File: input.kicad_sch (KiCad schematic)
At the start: 11 parts, among them J1 Conn_01x08

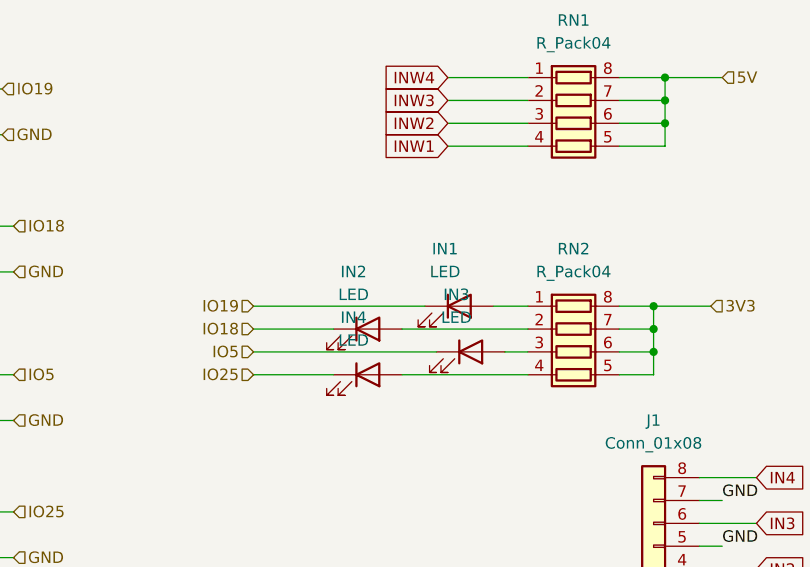
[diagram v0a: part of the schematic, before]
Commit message: 0
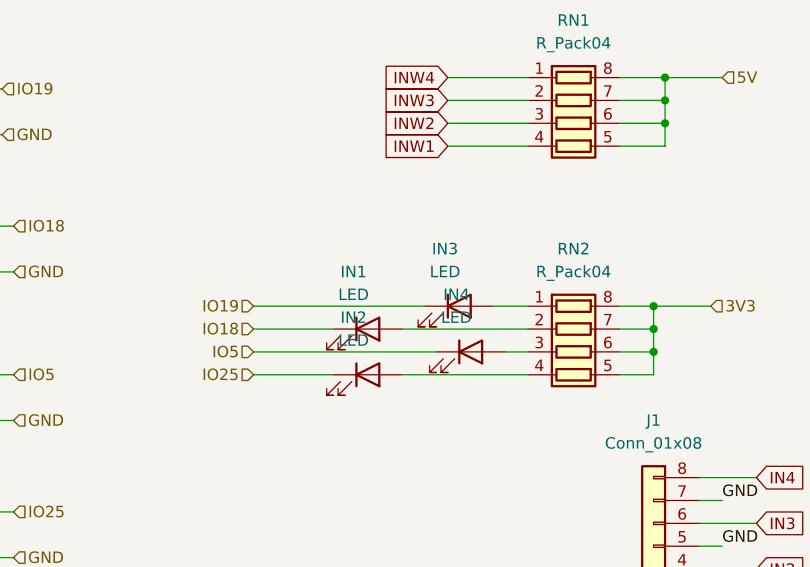
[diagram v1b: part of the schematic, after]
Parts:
- renumbered IN2 to IN1, IN4 to IN2, IN1 to IN3, IN3 to IN4
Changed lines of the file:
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@@
 		(pin "1"
+		)
+		(instances
+			(project "electronica"
+				(path "/a1c80da3-9403-4ec6-a34a-1db23a22b009/5b7b1883-0956-4642-a84a-0fce661aecfc"
+					(reference "OPT4")
+					(unit 1)
+				)
+			)
 		)
 	)
@@
 		(pin "1"
 		)
+		(instances
+			(project "electronica"
+				(path "/a1c80da3-9403-4ec6-a34a-1db23a22b009/5b7b1883-0956-4642-a84a-0fce661aecfc"
+					(reference "J1")
+					(unit 1)
+				)
+			)
+		)
 	)
 	(symbol
@@
 		(pin "8"
 		)
+		(instances
+			(project "electronica"
+				(path "/a1c80da3-9403-4ec6-a34a-1db23a22b009/5b7b1883-0956-4642-a84a-0fce661aecfc"
+					(reference "RN2")
+					(unit 1)
+				)
+			)
+		)
 	)
 	(symbol
@@
 		(pin "1"
 		)
+		(instances
+			(project "electronica"
+				(path "/a1c80da3-9403-4ec6-a34a-1db23a22b009/5b7b1883-0956-4642-a84a-0fce661aecfc"
+					(reference "OPT2")
+					(unit 1)
+				)
+			)
+		)
 	)
 	(symbol
@@
 		(pin "1"
 		)
+		(instances
+			(project "electronica"
+				(path "/a1c80da3-9403-4ec6-a34a-1db23a22b009/5b7b1883-0956-4642-a84a-0fce661aecfc"
+					(reference "OPT3")
+					(unit 1)
+				)
+			)
+		)
 	)
 	(symbol
@@
 		(dnp no)
 		(fields_autoplaced yes)
-		(property "Reference" "IN4"
+		(property "Reference" "IN2"
 			(at 171.1325 106.68 0)
 			(effects
@@
 		(pin "1"
 		)
+		(instances
+			(project "electronica"
+				(path "/a1c80da3-9403-4ec6-a34a-1db23a22b009/5b7b1883-0956-4642-a84a-0fce661aecfc"
+					(reference "IN2")
+					(unit 1)
+				)
+			)
+		)
 	)
 	(symbol
@@
 		(dnp no)
 		(fields_autoplaced yes)
-		(property "Reference" "IN1"
+		(property "Reference" "IN3"
 			(at 181.2925 99.06 0)
 			(effects
@@
 		(pin "1"
 		)
+		(instances
+			(project "electronica"
+				(path "/a1c80da3-9403-4ec6-a34a-1db23a22b009/5b7b1883-0956-4642-a84a-0fce661aecfc"
+					(reference "IN3")
+					(unit 1)
+				)
+			)
+		)
 	)
 	(symbol
@@
 		(dnp no)
 		(fields_autoplaced yes)
-		(property "Reference" "IN3"
+		(property "Reference" "IN4"
 			(at 182.5625 104.14 0)
 			(effects
@@
 		(pin "1"
 		)
+		(instances
+			(project "electronica"
+				(path "/a1c80da3-9403-4ec6-a34a-1db23a22b009/5b7b1883-0956-4642-a84a-0fce661aecfc"
+					(reference "IN4")
+					(unit 1)
+				)
+			)
+		)
 	)
 	(symbol
@@
 		(dnp no)
 		(fields_autoplaced yes)
-		(property "Reference" "IN2"
+		(property "Reference" "IN1"
 			(at 171.1325 101.6 0)
 			(effects
@@
 		(pin "1"
 		)
+		(instances
+			(project "electronica"
+				(path "/a1c80da3-9403-4ec6-a34a-1db23a22b009/5b7b1883-0956-4642-a84a-0fce661aecfc"
+					(reference "IN1")
+					(unit 1)
+				)
+			)
+		)
 	)
 	(symbol
@@
 		(pin "1"
 		)
+		(instances
+			(project "electronica"
+				(path "/a1c80da3-9403-4ec6-a34a-1db23a22b009/5b7b1883-0956-4642-a84a-0fce661aecfc"
+					(reference "OPT1")
+					(unit 1)
+				)
+			)
+		)
 	)
 	(symbol
@@
 		(pin "8"
 		)
-	)
+		(instances
+			(project "electronica"
+				(path "/a1c80da3-9403-4ec6-a34a-1db23a22b009/5b7b1883-0956-4642-a84a-0fce661aecfc"
+					(reference "RN1")
+					(unit 1)
+				)
+			)
+		)
+	)
